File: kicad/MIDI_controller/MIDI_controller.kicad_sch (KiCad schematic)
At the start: 15 parts, among them J1 AVR-ISP-6, J2 DIN-5, J3 Jack-DC, SW1 RotaryEncoder_Switch, U1 ATmega328P-P, U2 MCP23017_SP, U3 MCP23017_SP, U4 MCP23017_SP, U5 LM317_TO-220, Y1 Crystal

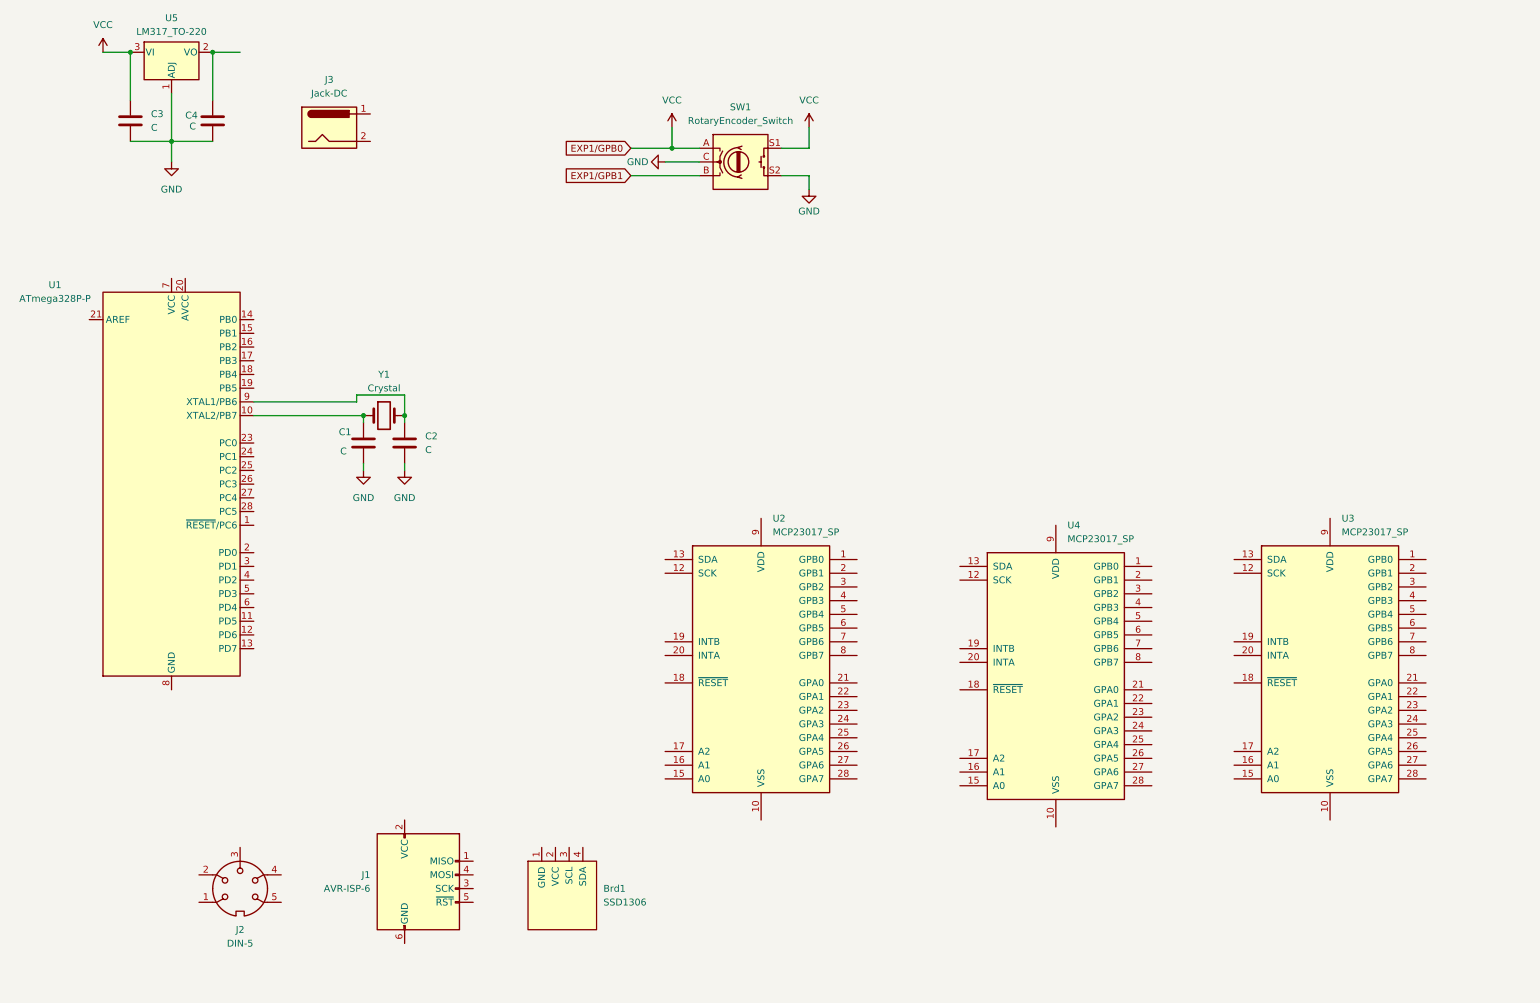
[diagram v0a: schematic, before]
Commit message: update kicad schematic
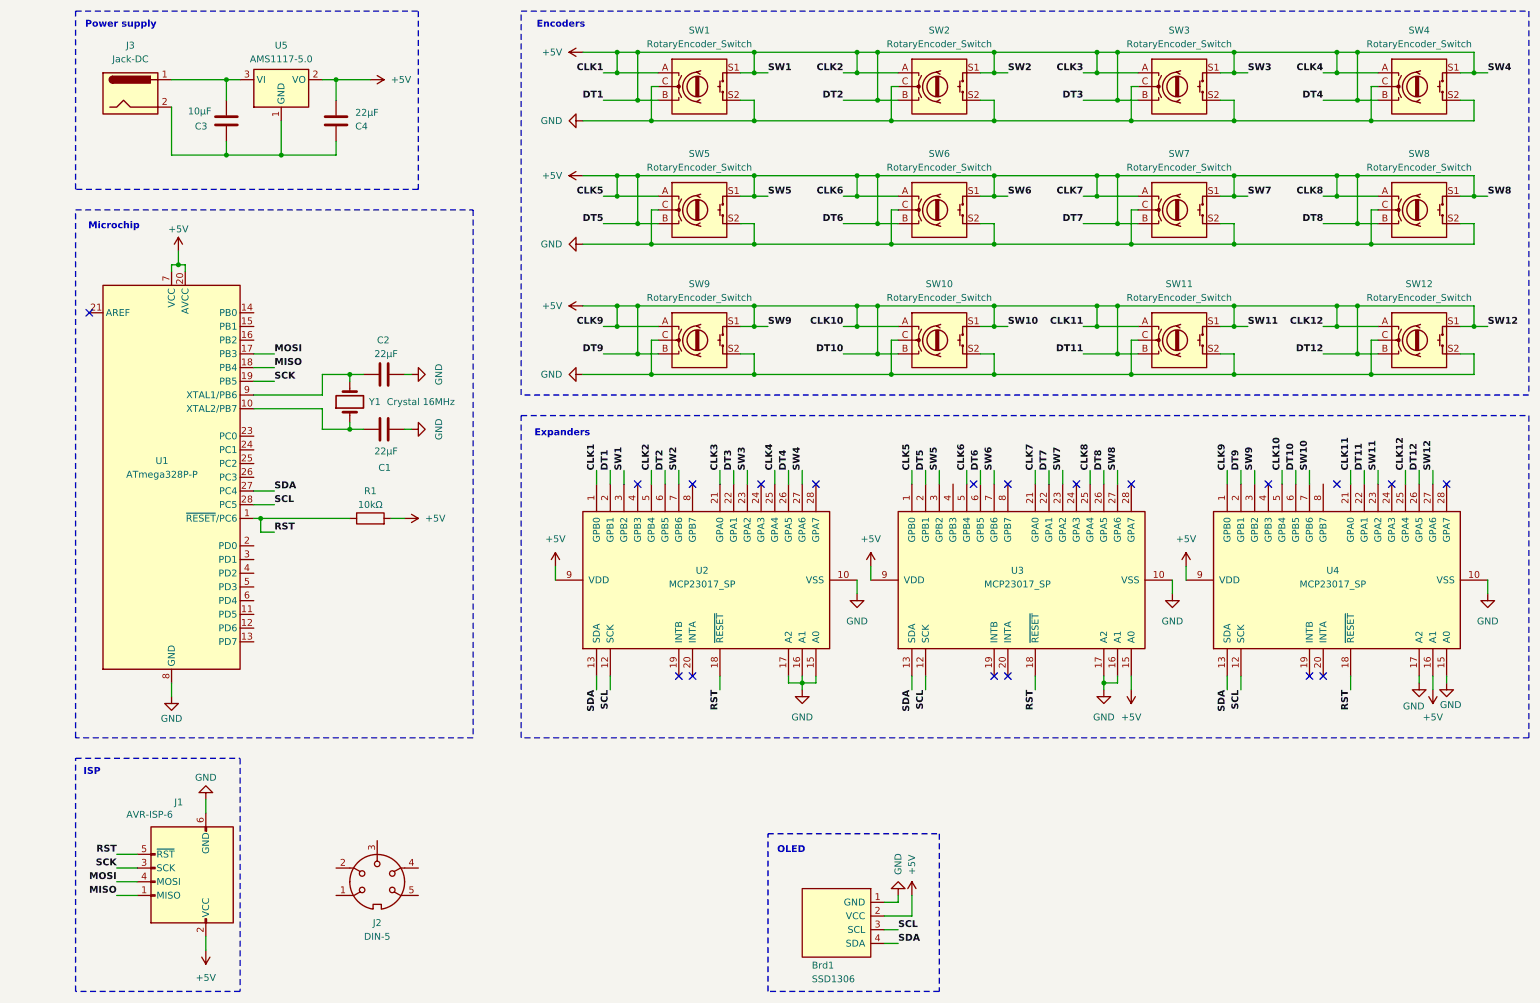
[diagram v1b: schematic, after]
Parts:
- removed U5: LM317_TO-220, Package_TO_SOT_THT:TO-220-3_Vertical, symbol Regulator_Linear:LM317_TO-220
- added R1: 10kΩ, symbol Device:R
- added SW10, SW11, SW12, SW2, SW3, SW4, SW5, SW6, SW7, SW8, SW9: RotaryEncoder_Switch, symbol Device:RotaryEncoder_Switch
- added U5: AMS1117-5.0, Package_TO_SOT_SMD:SOT-223-3_TabPin2, symbol Regulator_Linear:AMS1117-5.0
- C1, C2, C4: value C -> 22μF
- C3: value C -> 10μF
- Y1: value Crystal -> Crystal 16MHz
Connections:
- net EXP1/GPB1 is gone; now on net +5V: SW1.B
- net GND: now also Brd1.1 (GND), J1.6 (GND), U1.22 (GND), U1.8 (GND), U2.10 (VSS), U2.15 (A0), U2.16 (A1), U2.17 (A2), U3.10 (VSS), U3.16 (A1), U3.17 (A2), U4.10 (VSS), U4.15 (A0), U4.17 (A2), SW10.C, SW10.S2, SW11.C, SW11.S2, SW12.C, SW12.S2, SW2.C, SW2.S2, SW3.C, SW3.S2, SW4.C, SW4.S2, SW5.C, SW5.S2, SW6.C, SW6.S2, SW7.C, SW7.S2, SW8.C, SW8.S2, SW9.C, SW9.S2; no longer C3.2, C4.2
- net +5V: now reaches C4.1
- net +5V: now also Brd1.2 (VCC), J1.2 (VCC), SW1.A, SW1.S1, U1.20 (AVCC), U1.7 (VCC), U2.1 (GPB0), U2.2 (GPB1), U2.21 (GPA0), U2.22 (GPA1), U2.23 (GPA2), U2.25 (GPA4), U2.26 (GPA5), U2.27 (GPA6), U2.3 (GPB2), U2.5 (GPB4), U2.6 (GPB5), U2.7 (GPB6), U2.9 (VDD), U3.1 (GPB0), U3.15 (A0), U3.2 (GPB1), U3.21 (GPA0), U3.22 (GPA1), U3.23 (GPA2), U3.25 (GPA4), U3.26 (GPA5), U3.27 (GPA6), U3.3 (GPB2), U3.5 (GPB4), U3.6 (GPB5), U3.7 (GPB6), U3.9 (VDD), U4.1 (GPB0), U4.16 (A1), U4.2 (GPB1), U4.21 (GPA0), U4.22 (GPA1), U4.23 (GPA2), U4.25 (GPA4), U4.26 (GPA5), U4.27 (GPA6), U4.3 (GPB2), U4.5 (GPB4), U4.6 (GPB5), U4.7 (GPB6), U4.9 (VDD), R1.2, SW10.A, SW10.B, SW10.S1, SW11.A, SW11.B, SW11.S1, SW12.A, SW12.B, SW12.S1, SW2.A, SW2.B, SW2.S1, SW3.A, SW3.B, SW3.S1, SW4.A, SW4.B, SW4.S1, SW5.A, SW5.B, SW5.S1, SW6.A, SW6.B, SW6.S1, SW7.A, SW7.B, SW7.S1, SW8.A, SW8.B, SW8.S1, SW9.A, SW9.B, SW9.S1, U5.2 (VO)
- net RST: now reaches U1.1 (~{RESET}/PC6)
- net RST: now also J1.5 (~{RST}), U2.18 (~{RESET}), U3.18 (~{RESET}), U4.18 (~{RESET}), R1.1
- net MOSI: now reaches U1.17 (PB3)
- net MOSI: now also J1.4 (MOSI)
- net MISO: now reaches U1.18 (PB4)
- net MISO: now also J1.1 (MISO)
- net SCK: now reaches U1.19 (PB5)
- net SCK: now also J1.3 (SCK)
- net SDA: now reaches U1.27 (PC4)
- net SDA: now also Brd1.4 (SDA), U2.13 (SDA), U3.13 (SDA), U4.13 (SDA)
- net SCL: now reaches U1.28 (PC5)
- net SCL: now also Brd1.3 (SCL), U2.12 (SCK), U3.12 (SCK), U4.12 (SCK)
- net at J3.1: now also C3.1, U5.3 (VI)
- net at J3.2: now also C3.2, C4.2, U5.1 (GND)
- removed net VCC: C3.1, SW1.A, SW1.S1
- no-connect marks 0 -> 19
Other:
- note added: "Encoders"
- note added: "Expanders"
- note added: "ISP"
- note added: "Microchip"
- note added: "OLED"
- note added: "Power supply"
- title: (none) -> MIDI Controller
- moved on the sheet: Brd1, C1, C2, C3, C4, J1, J2, J3, SW1, U1, U2, Y1
